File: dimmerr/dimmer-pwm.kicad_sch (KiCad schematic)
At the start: 2 parts, among them Q1 TIP41C

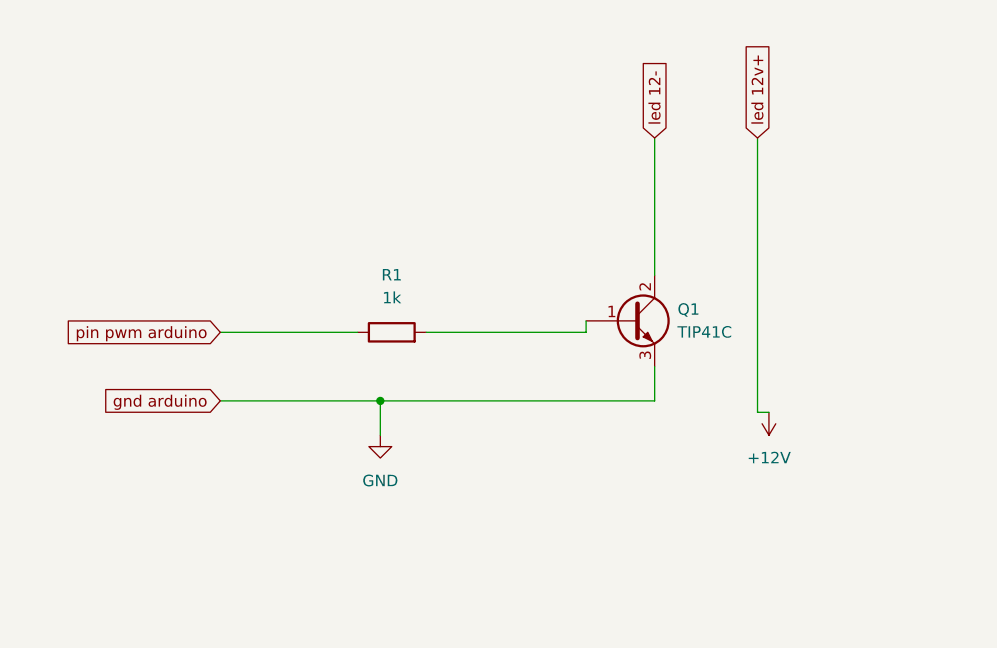
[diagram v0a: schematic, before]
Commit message: cicuito
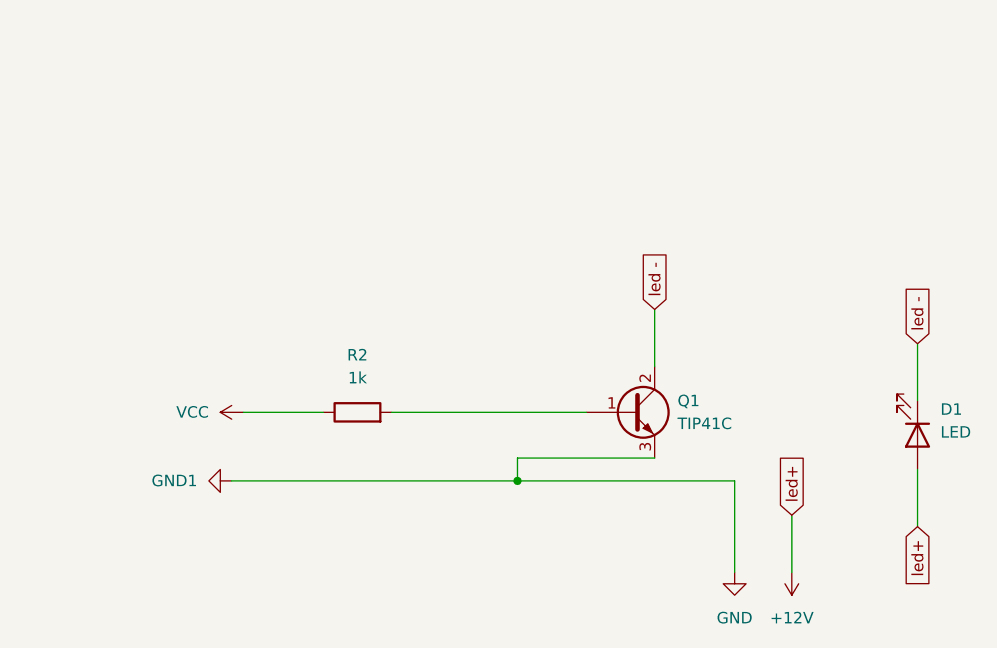
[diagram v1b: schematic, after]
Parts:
- removed R1: 1k, symbol Device:R
- added D1: LED, LED_THT:LED_D5.0mm_Clear, symbol Device:LED
- added R2: 1k, Resistor_THT:R_Axial_DIN0204_L3.6mm_D1.6mm_P5.08mm_Horizontal, symbol Device:R
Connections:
- net +12V: now also D1.2 (A)
- net at Q1.1 (B): now also R2.2
- net led 12- renamed led -
- net led -: now also D1.1 (K)
- new net VCC: R2.1
